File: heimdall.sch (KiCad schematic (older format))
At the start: 15 parts, among them P1 CONN, U1 ESP-01, U2 TLP222A, U3 UA78M33CDCY

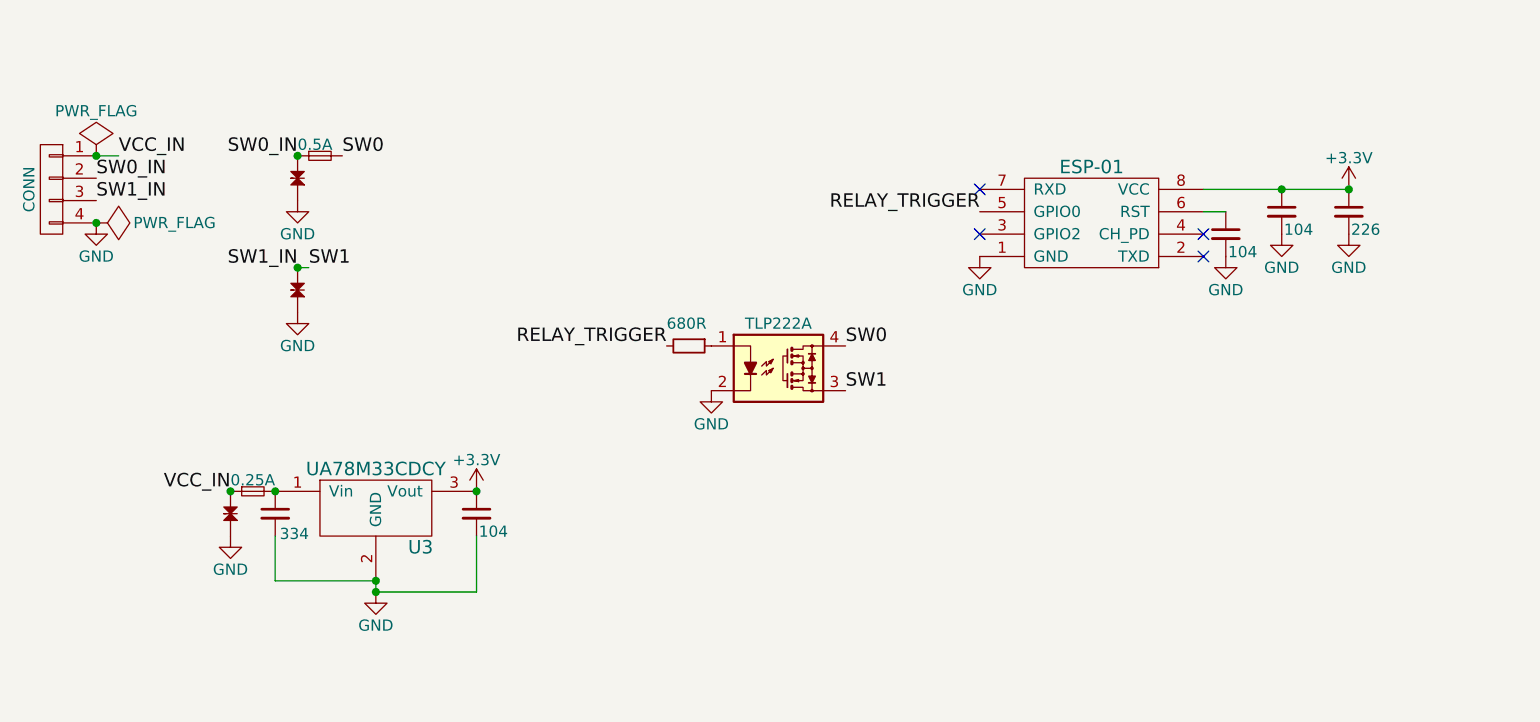
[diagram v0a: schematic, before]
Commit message: Much faffing, many switch mode supply, very PCB.
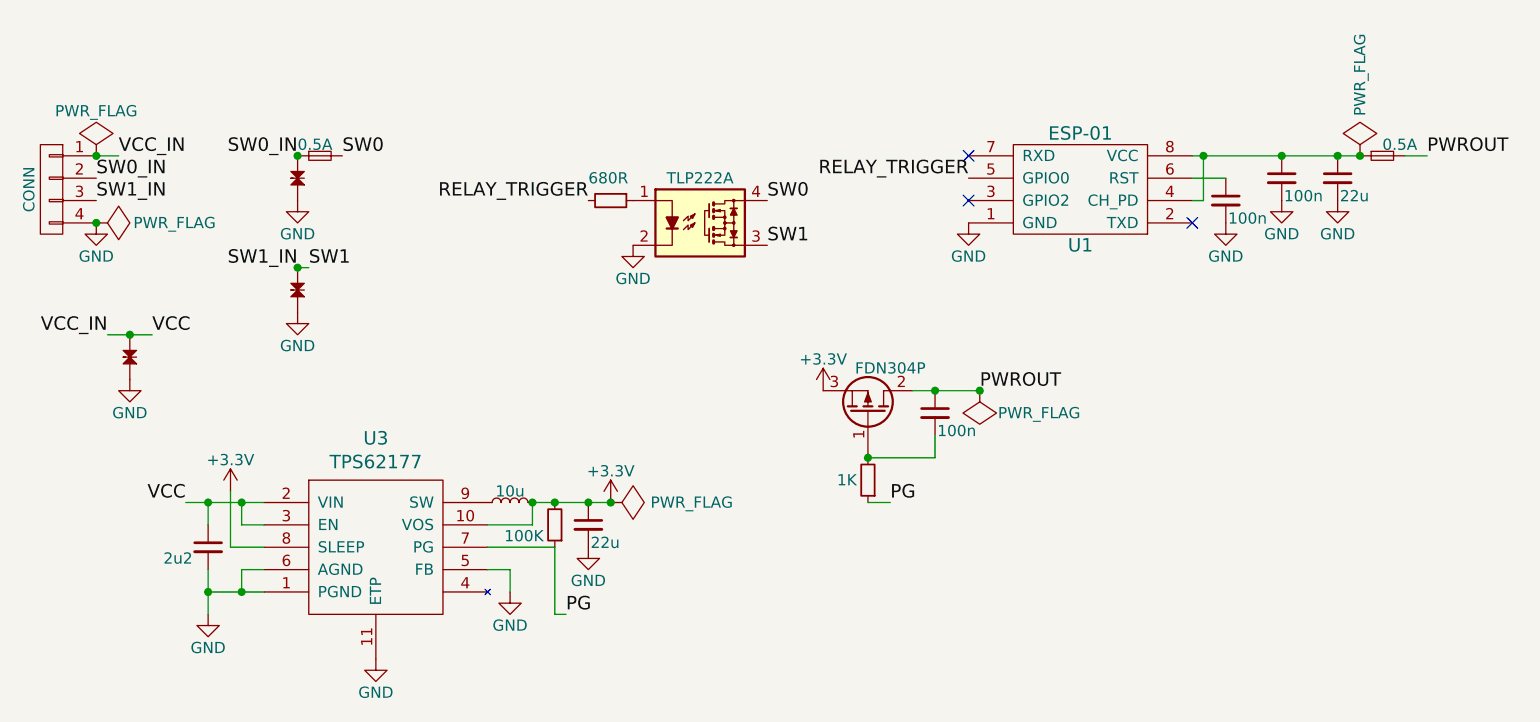
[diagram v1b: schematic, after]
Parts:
- removed U3: UA78M33CDCY, TO_SOT_Packages_SMD:SOT-223, symbol UA78M33CDCY
- added C6: 2u2, Capacitors_SMD:C_0603, symbol C_Small
- added L1: 10u, Wurth:WE-TPC, symbol L_Small
- added Q1: FDN304P, Housings_SSOT:SuperSOT-3, symbol Q_PMOS_GDS
- added R2: 100K, Resistors_SMD:R_0603, symbol R_Small
- added R3: 1K, Resistors_SMD:R_0603, symbol R_Small
- added U3: TPS62177, Housing_WSON:WSON-10, symbol TPS62177
- C1: value 334 -> 22u; Farnell 2496926 -> 2496833
- C2, C3, C4: value 104 -> 100n
- C5: value 226 -> 22u; footprint Capacitors_SMD:C_1206 -> Capacitors_SMD:C_0603
- F2: value 0.25A -> 0.5A; Farnell 9921826 -> 9921834
- R1: footprint Resistors_SMD:R_0603 -> Resistors_SMD:R_1206
- U1: footprint Socket_Strips:Socket_Strip_Straight_2x04 -> esp:ESP-01-NoSilk
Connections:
- net +3V3: now also C1.1, L1.2, Q1.3 (S), R2.2, U3.10 (VOS), U3.8 (SLEEP); no longer C2.1, C4.1, C5.1, U1.8 (VCC)
- net GND: now also C6.2, U3.1 (PGND), U3.11 (ETP), U3.5 (FB), U3.6 (AGND); no longer C2.2
- net at U1.4 (CH_PD): now also C4.1, C5.1, F2.1, U1.8 (VCC)
- net PWROUT: now reaches F2.2
- net PWROUT: now also C2.1, Q1.2 (D); no longer C1.1
- net VCC_IN renamed VCC
- net VCC: now also C6.1, U3.2 (VIN), U3.3 (EN); no longer F2.1
- new net: L1.1, U3.9 (SW)
- new net: C2.2, Q1.1 (G), R3.2
- new net PG: R2.1, R3.1, U3.7 (PG)
- no-connect marks 4 -> 3

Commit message: Various shuffling
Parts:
- R1: footprint Resistors_SMD:R_1206 -> Resistors_SMD:R_0603
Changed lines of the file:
@@
 F 0 "R1" H 3180 970 50  0001 L CNN
 F 1 "680R" V 3050 850 50  0000 L CNN
-F 2 "Resistors_SMD:R_1206" H 3150 950 50  0001 C CNN
+F 2 "Resistors_SMD:R_0603" H 3150 950 50  0001 C CNN
 F 3 "" H 3150 950 50  0000 C CNN
 	1    3150 950
